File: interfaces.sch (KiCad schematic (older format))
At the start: 0 parts

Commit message: update,
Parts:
- added U?: FC-40P-LCD, symbol taobao-components:FC-40P-LCD
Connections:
- net labels added: +3V3, GND, LCD_CLK, LCD_D10, LCD_D11, LCD_D12, LCD_D13, LCD_D14, LCD_D15, LCD_D18, LCD_D19, LCD_D2, LCD_D20, LCD_D21, LCD_D22, LCD_D23, LCD_D3, LCD_D4, LCD_D5, LCD_D6, LCD_D7, LCD_DE, LCD_HSYNC, LCD_VSYNC, TPX1, TPX2, TPY1, TPY2, VLED+, VLED-
- wire segments 0 -> 52

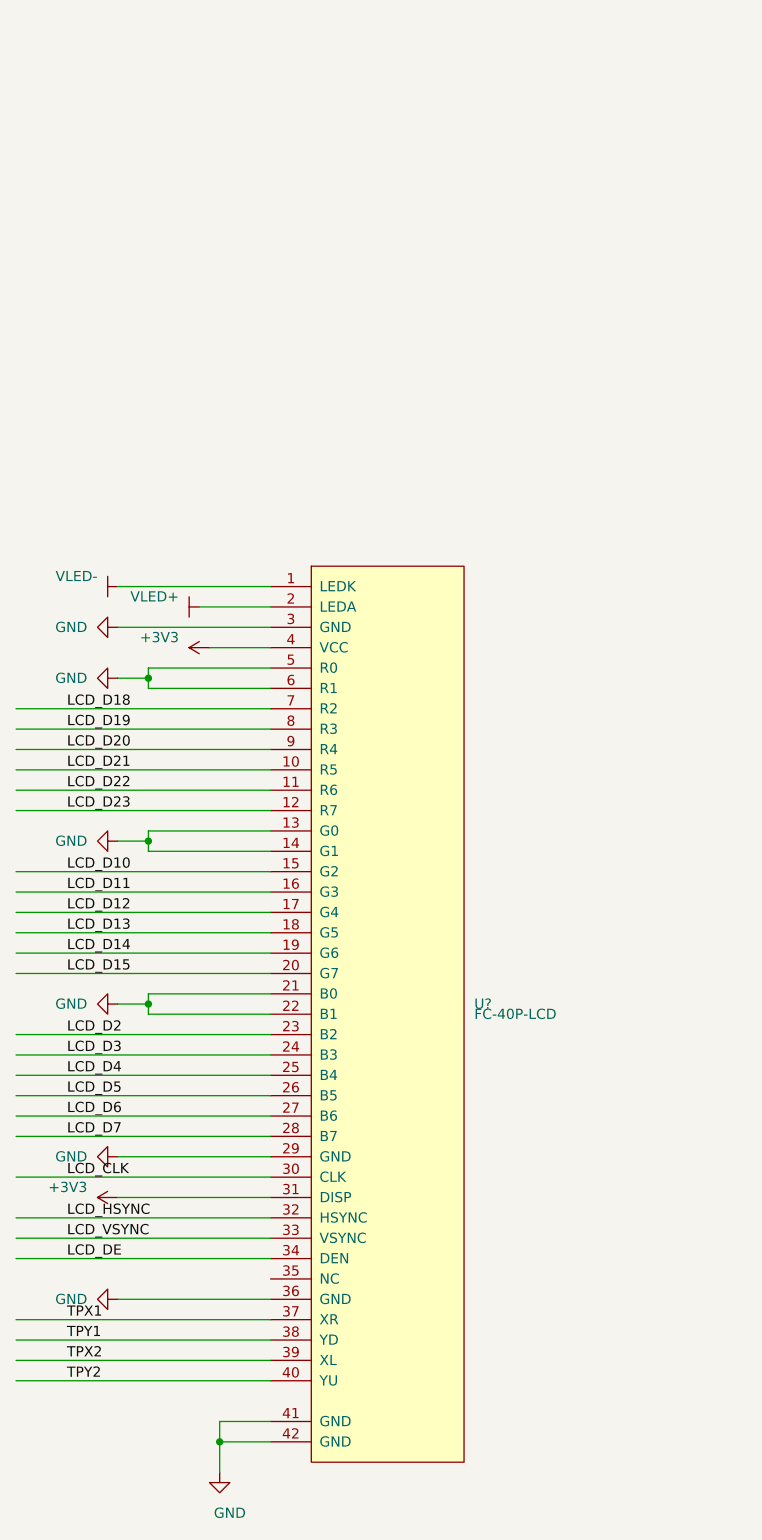
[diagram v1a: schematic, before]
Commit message: update,
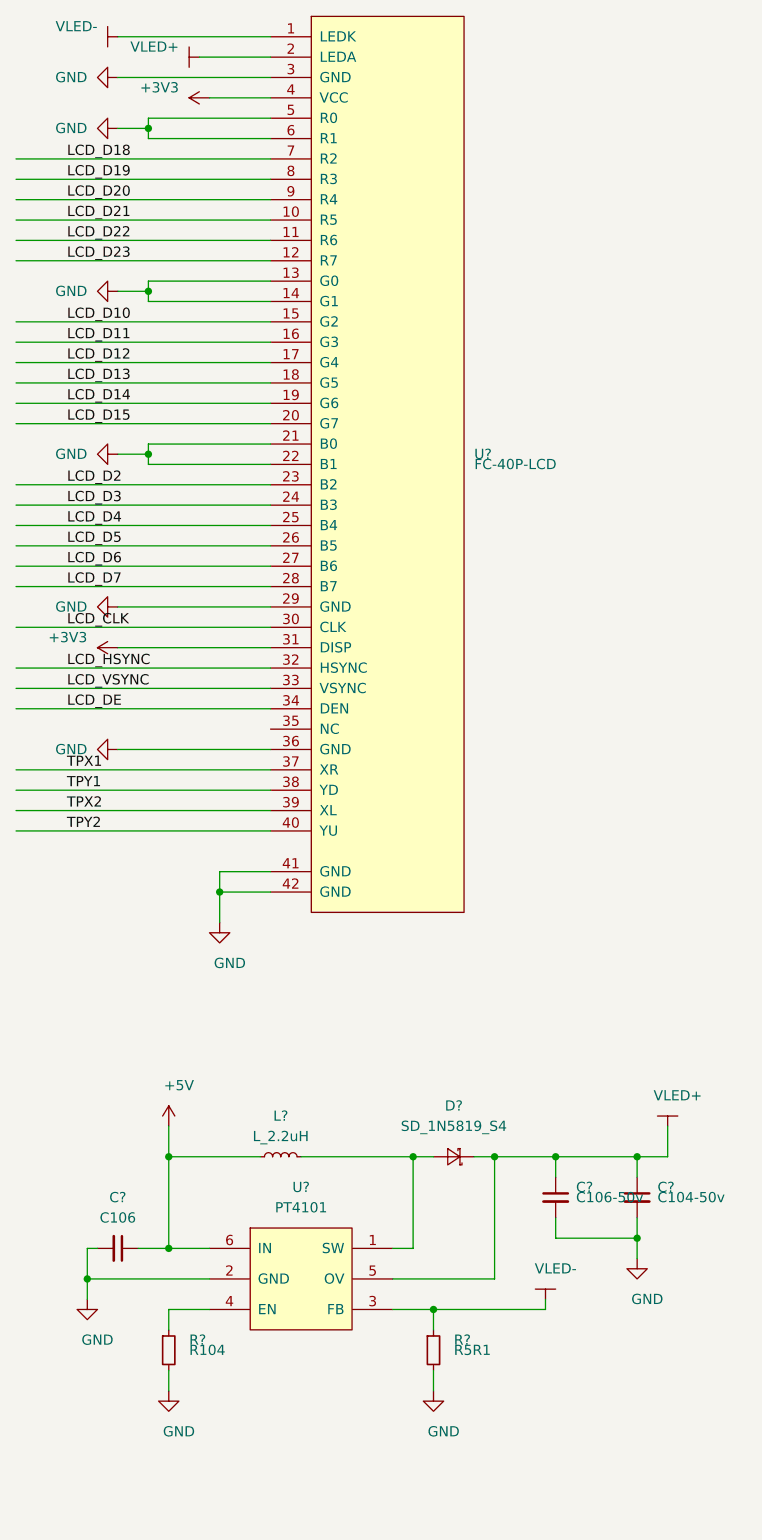
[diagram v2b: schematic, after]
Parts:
- added C?: C106, symbol taobao-c:C106
- added C?: C106-50v, symbol taobao-c:C106-50v
- added C?: C104-50v, symbol taobao-c:C104-50v
- added D?: SD_1N5819_S4, symbol taobao-sd:SD_1N5819_S4
- added L?: L_2.2uH, symbol taobao-l:L_2.2uH
- added R?: R104, symbol taobao-r:R104
- added R?: R5R1, symbol taobao-r:R5R1
- added U?: PT4101, symbol taobao-components:PT4101
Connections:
- net labels added: +5V
- wire segments 52 -> 86
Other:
- moved on the sheet: U?
